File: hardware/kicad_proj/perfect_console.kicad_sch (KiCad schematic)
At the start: 73 parts, among them J1 R_Out, J10 PWR_OUT_Pins, J11 GPIO5-7, J12 USB_Out, J13 I2C, J14 ESP_UART, J15 GPIO41, J16 CH_UART, J17 CH_Flash, J18 Micro_SD_Card, J2 Jack_3.5, J3 L_Out, J4 USB, J5 TP4056_WO_Protect, J6 Bat, J7 PWR_Btn, J8 BTN_Pins, J9 PTT_Btn, Q1 NMOS, Q2 NMOS, Q3 NMOS, Q4 NMOS, Q5 NMOS, Q6 NMOS, SW1 Reset, SW2 Boot, U1 ESP32-S3-WROOM1, U2 Display, U3 PCM5102, U4 PAM8403, U5 CH32V006E8R6, U6 LoRa, U7 USBLC6-2SC6, U8 Mic, U9 DC-DC

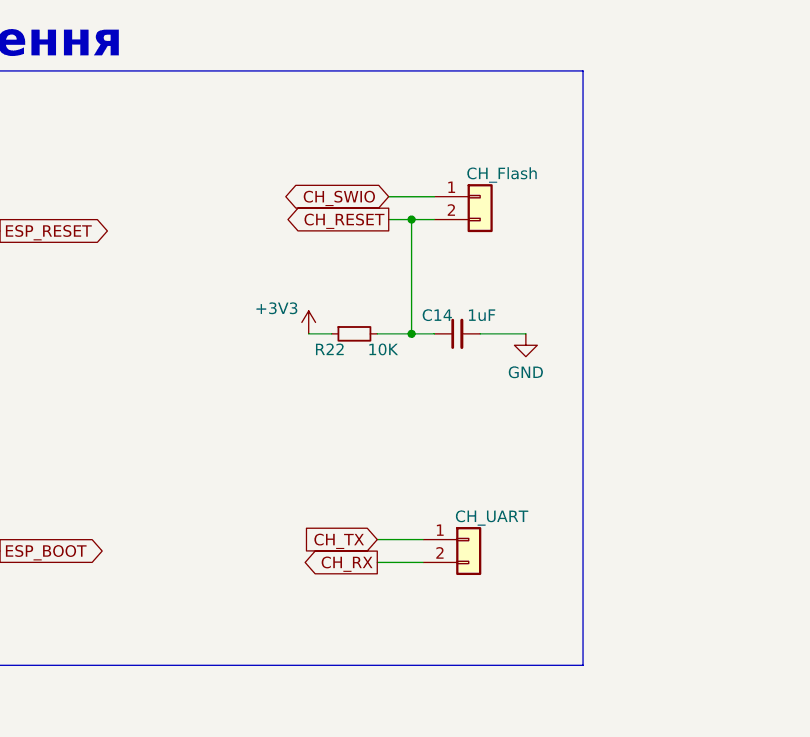
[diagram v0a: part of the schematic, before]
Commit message: Доопрацювання схеми
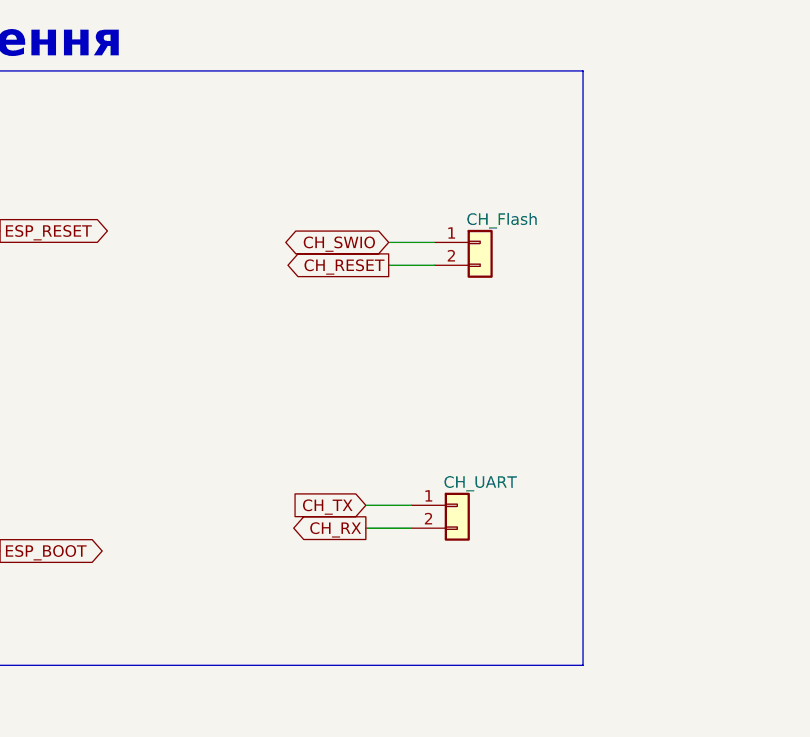
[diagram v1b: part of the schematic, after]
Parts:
- removed C14: 1uF, Capacitor_SMD:C_1206_3216Metric, symbol Device:C_Small
- removed R22: 10K, Resistor_SMD:R_1206_3216Metric_Pad1.30x1.75mm_HandSolder, symbol Device:R_Small
